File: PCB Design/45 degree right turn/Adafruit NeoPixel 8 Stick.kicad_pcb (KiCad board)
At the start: 2 copper layers, 26 x 21.4 mm, 4 parts, among them CN1 1X4SMT, CN2 1X4SMT

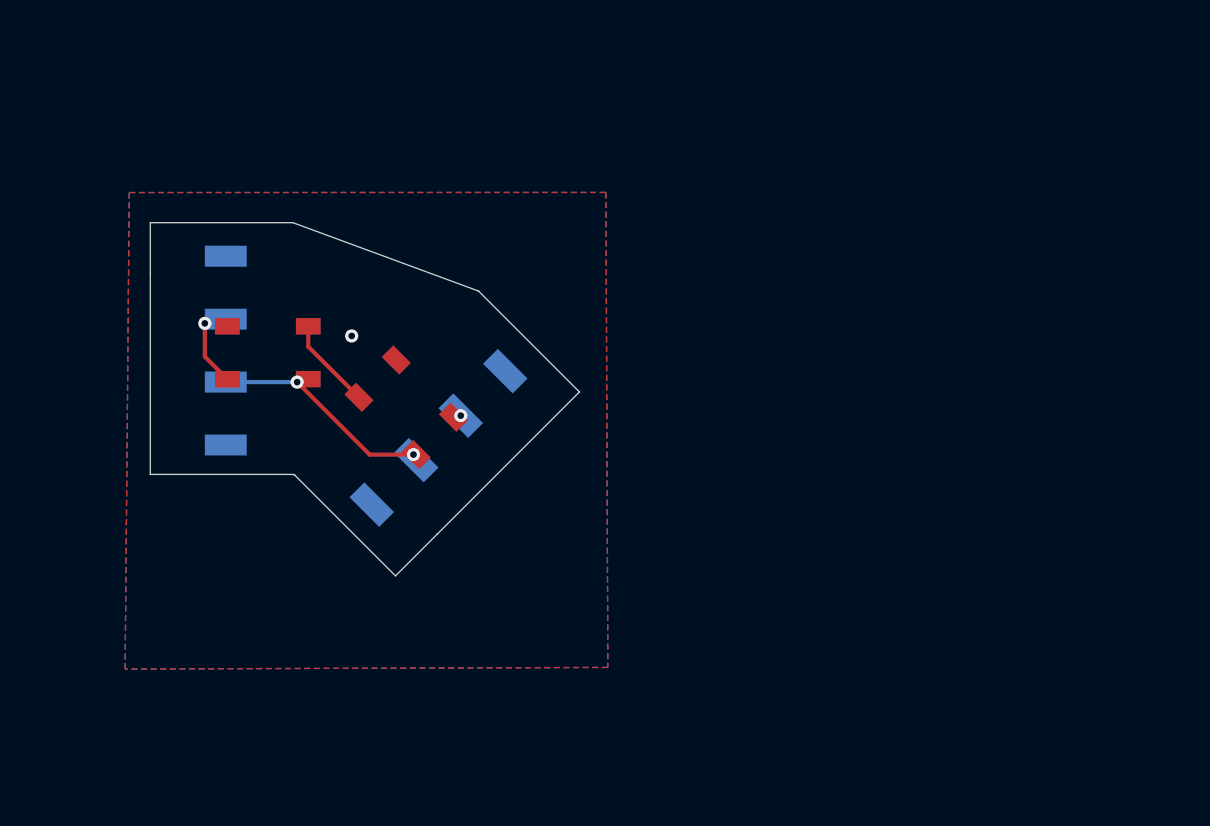
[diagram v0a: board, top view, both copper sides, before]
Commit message: 6 pin
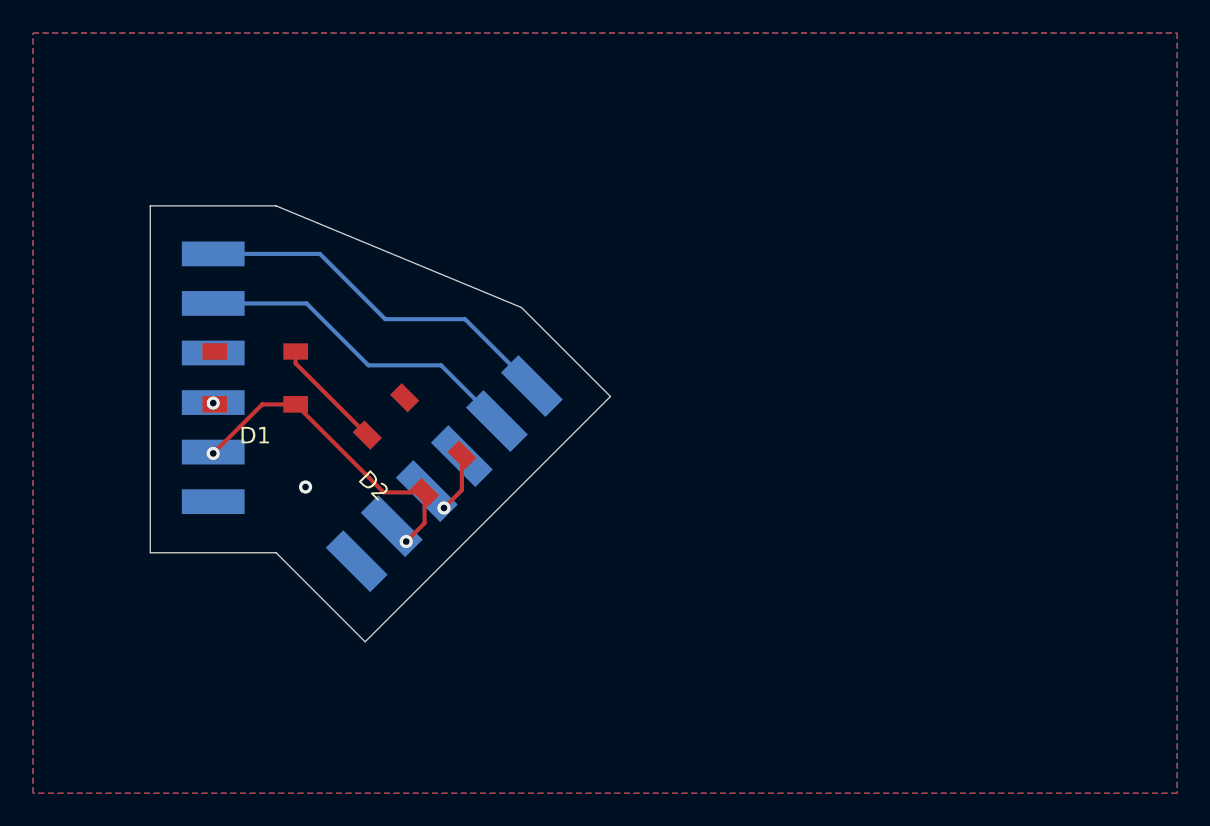
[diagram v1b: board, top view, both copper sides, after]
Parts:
- moved CN1 2.67 mm to (139.4, 113.6)
- moved D2 2.34 mm to (138.4, 112.0)
- moved D1 1.70 mm to (128.8, 108.0)
- moved CN2 0.52 mm to (126.9, 107.4)
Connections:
- CN1 pad 1: GND -> Net-(CN1-Pad1)
- CN1 pad 2: Net-(D2-Pad2) -> Net-(CN1-Pad2)
- CN1 pad 3: +5V -> GND
- CN1 pad 4: GND -> Net-(CN1-Pad4)
- D2 pad 2: Net-(D2-Pad2) -> Net-(CN1-Pad4)
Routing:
- net Net-(CN1-Pad1): track 0.00 -> 22.6 mm
- net Net-(CN1-Pad2): track 0.00 -> 20.1 mm
- net +5V: track 13.3 -> 19.7 mm
- net Net-(CN2-Pad3): track 3.94 -> 0.00 mm
- net Net-(CN1-Pad4): track 0.00 -> 3.66 mm, vias 0 -> 1
- net Net-(D1-Pad2): track 5.57 -> 6.86 mm
- net Net-(D2-Pad2): vias 1 -> 0
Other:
- board size 26 x 21.4 mm -> 27.9 x 26.4 mm
- board text removed: "4-7VDC"
- board text removed: "DOUT"
- board text removed: "GND"
